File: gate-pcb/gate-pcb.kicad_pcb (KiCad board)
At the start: 2 copper layers, 21 x 25.5 mm, 6 parts, among them J1 EXT_IN, J2 EXT_OUT, J3 LED_START, J4 LED_END

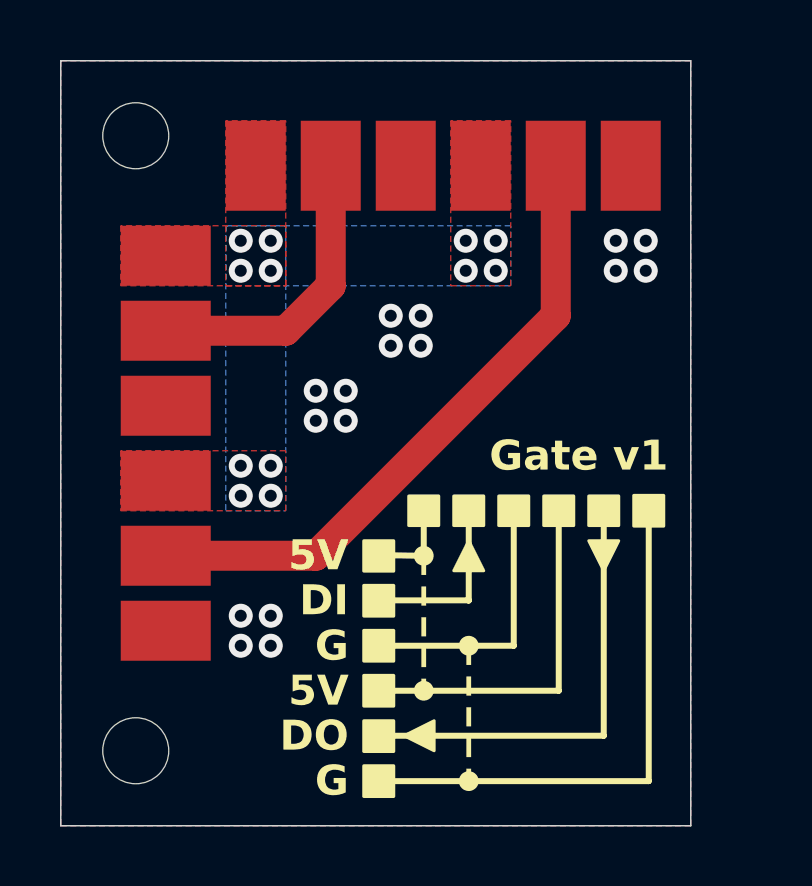
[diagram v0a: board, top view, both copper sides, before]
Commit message: v1
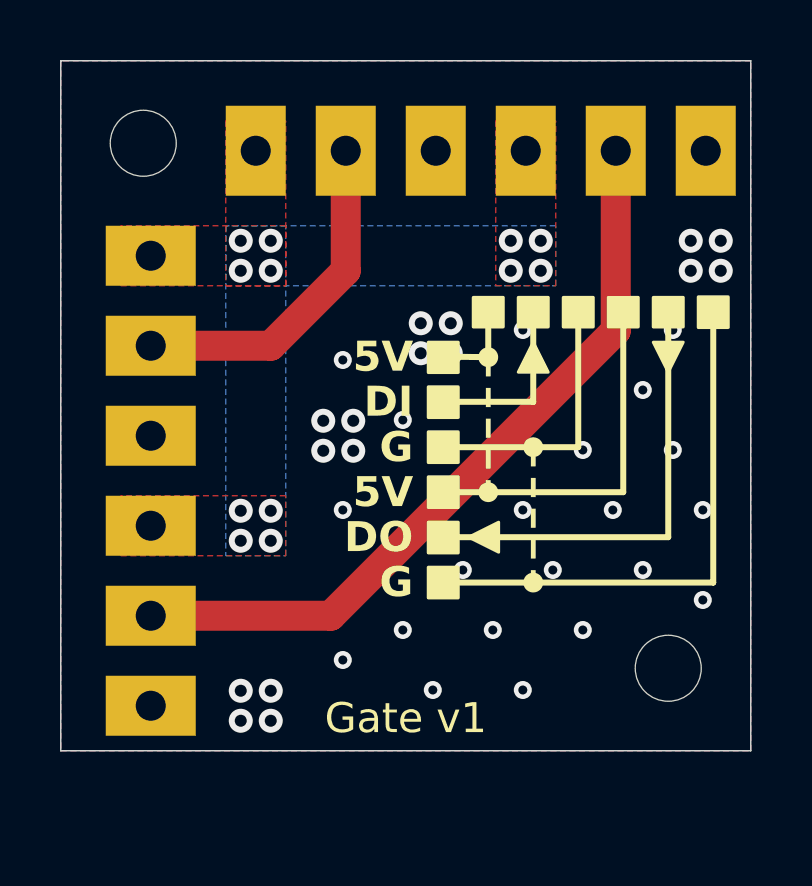
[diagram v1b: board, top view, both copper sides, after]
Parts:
- moved REF** 18.0 mm to (124.8, 53.2)
- moved J2 2.06 mm to (107.5, 51.5)
- moved J4 2.06 mm to (123.0, 36.0)
- moved J1 0.71 mm to (107.5, 42.5)
- moved J3 0.71 mm to (114.0, 36.0)
- moved REF** 0.35 mm to (107.2, 35.8)
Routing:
- net Net-(J2-DATA_OUT): track 21.3 -> 25.4 mm
- net Net-(J1-DATA_IN): track 10.1 -> 11.5 mm
- net Net-(J1-GND): vias 16 -> 37
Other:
- board size 21 x 25.5 mm -> 23 x 23 mm
